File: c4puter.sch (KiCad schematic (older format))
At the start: 19 parts, among them J7 19V 3A, Q1 AOD4189, Q2 AOD4189, SW1 POWER, SW2 SW

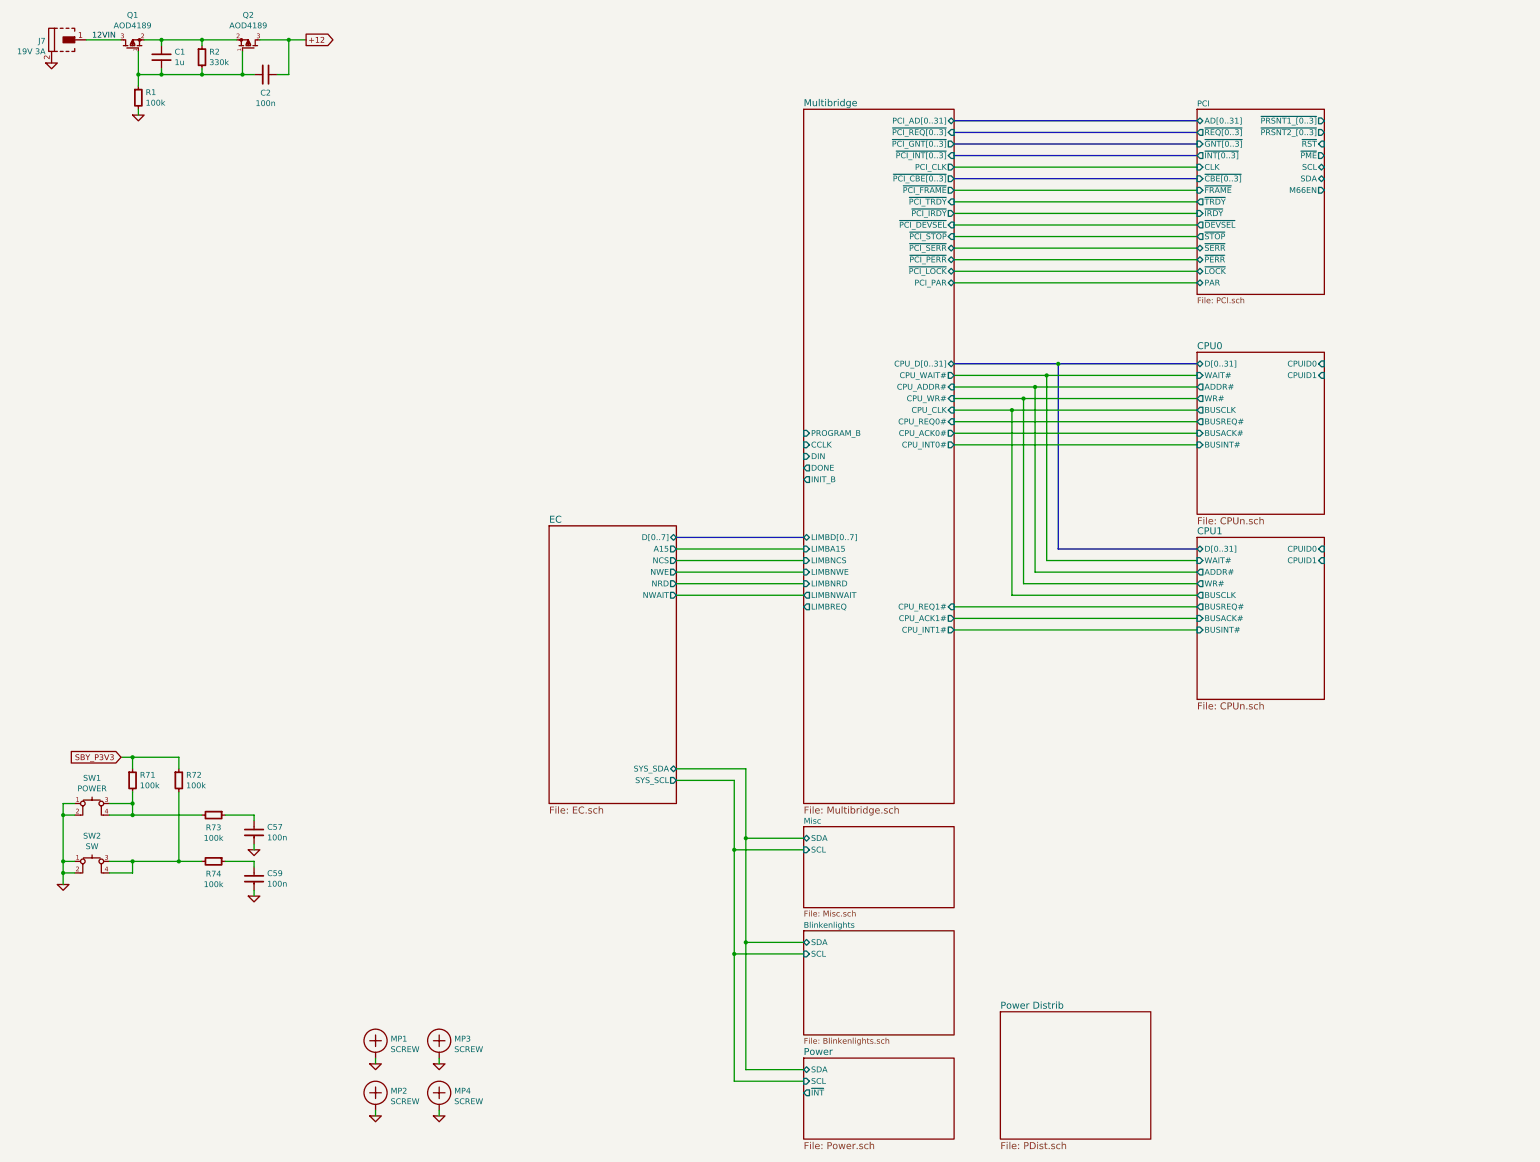
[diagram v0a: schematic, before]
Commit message: TODO: learn to write good commit messages
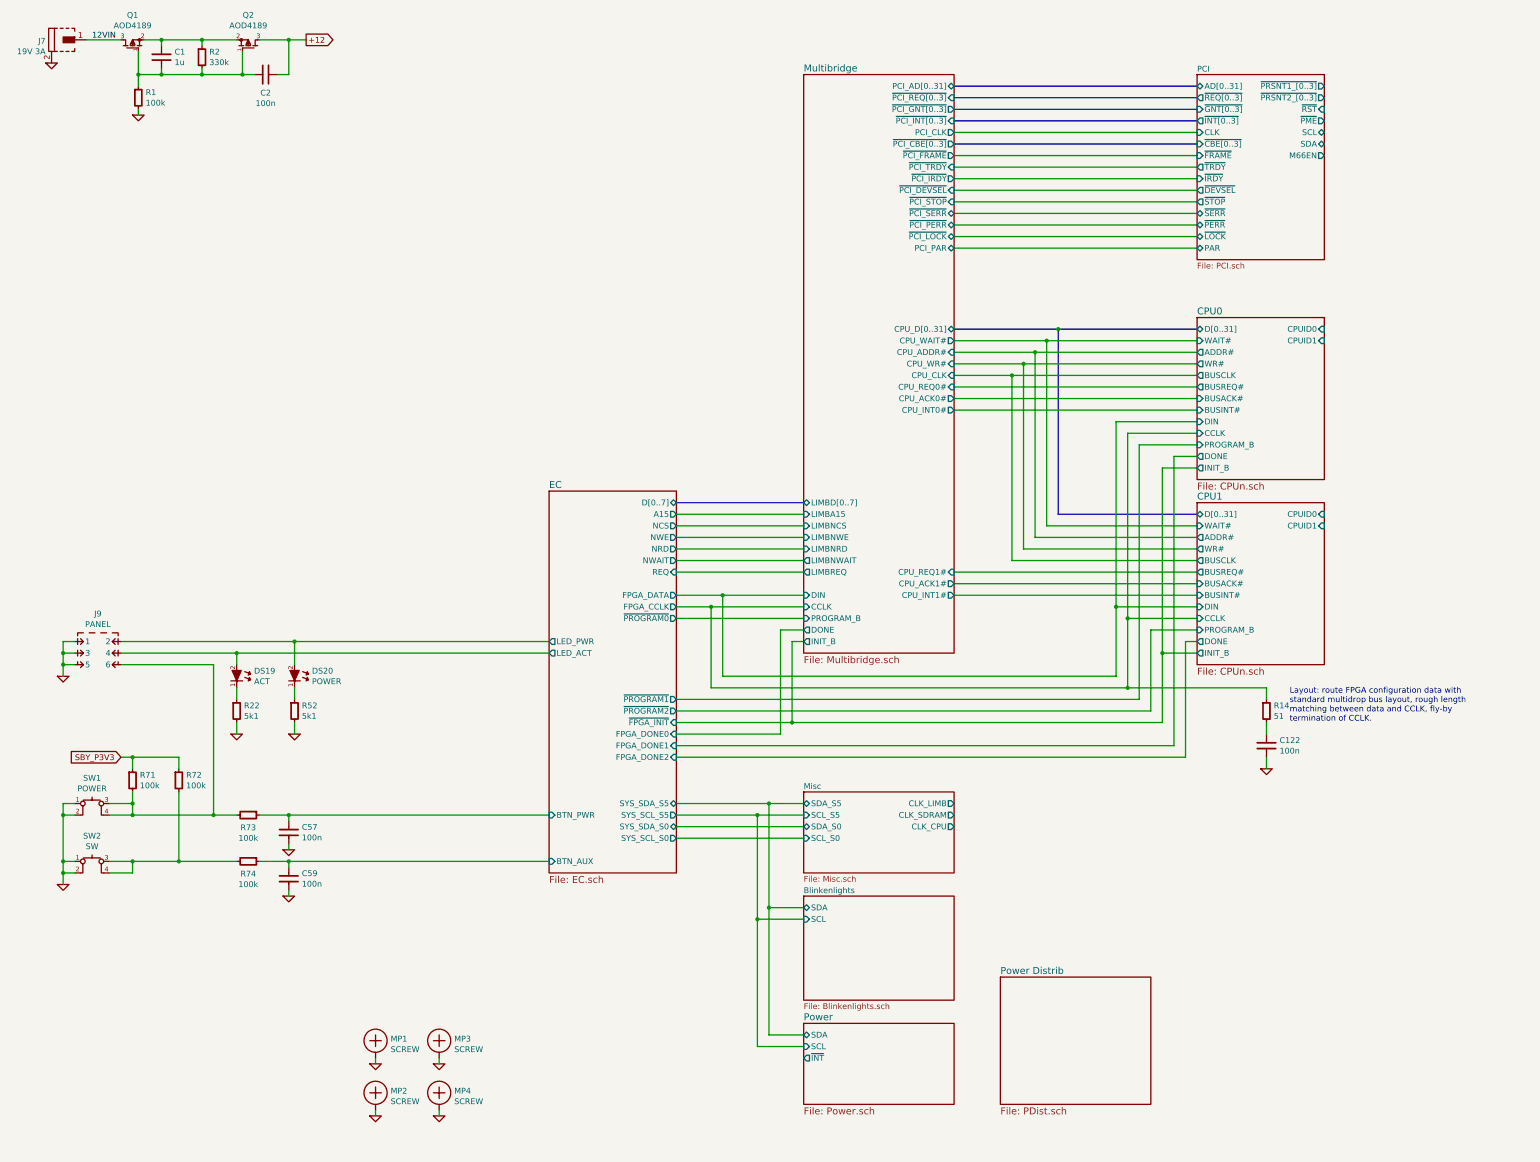
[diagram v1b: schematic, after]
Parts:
- added C122: 100n, IPC7351-Nominal:CAPC1005X55, symbol C-0402
- added DS19: ACT, smd-semi:LED-0603, symbol LED-0603
- added DS20: POWER, smd-semi:LED-0603, symbol LED-0603
- added J9: PANEL, conn-100mil:CONN-100MIL-M-2x3, symbol CONN-100MIL-M-2x3
- added R14: 51, IPC7351-Nominal:RESC1005X40, symbol R-0402
- added R22, R52: 5k1, IPC7351-Nominal:RESC1005X40, symbol R-0402
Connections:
- net GND: now also C122.2, J9.1, J9.3, J9.5, R22.2, R52.2
- net at R71.2, R73.2, SW1.3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: now also J9.6
- net EC/BTN_PWR: now reaches C57.1, R73.1
- net EC/BTN_AUX: now reaches C59.1, R74.1
- new net: C122.1, R14.2
- new net: DS20.1 (K), R52.1
- new net: DS19.1 (K), R22.1
- new net CPU0/CCLK: R14.1
- new net EC/LED_ACT: DS19.2 (A), J9.4
- new net EC/LED_PWR: DS20.2 (A), J9.2
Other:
- note added: "Layout: route FPGA configuration data with\nstandard multidrop bus layout, rough length\nmatching between data and CCLK, fly-by\ntermination of CCLK."
- moved on the sheet: C57, C59, R73, R74
